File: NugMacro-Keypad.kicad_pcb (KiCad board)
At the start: 2 copper layers, 76.2 x 97.2 mm, 51 parts, among them J2 Conn_01x04, J3 Conn_01x04_Female_For_LCD, SW1 SW_Push, SW2 RotaryEncoder_Switch, U1 ATmega32U4-A, Y1 16MHz

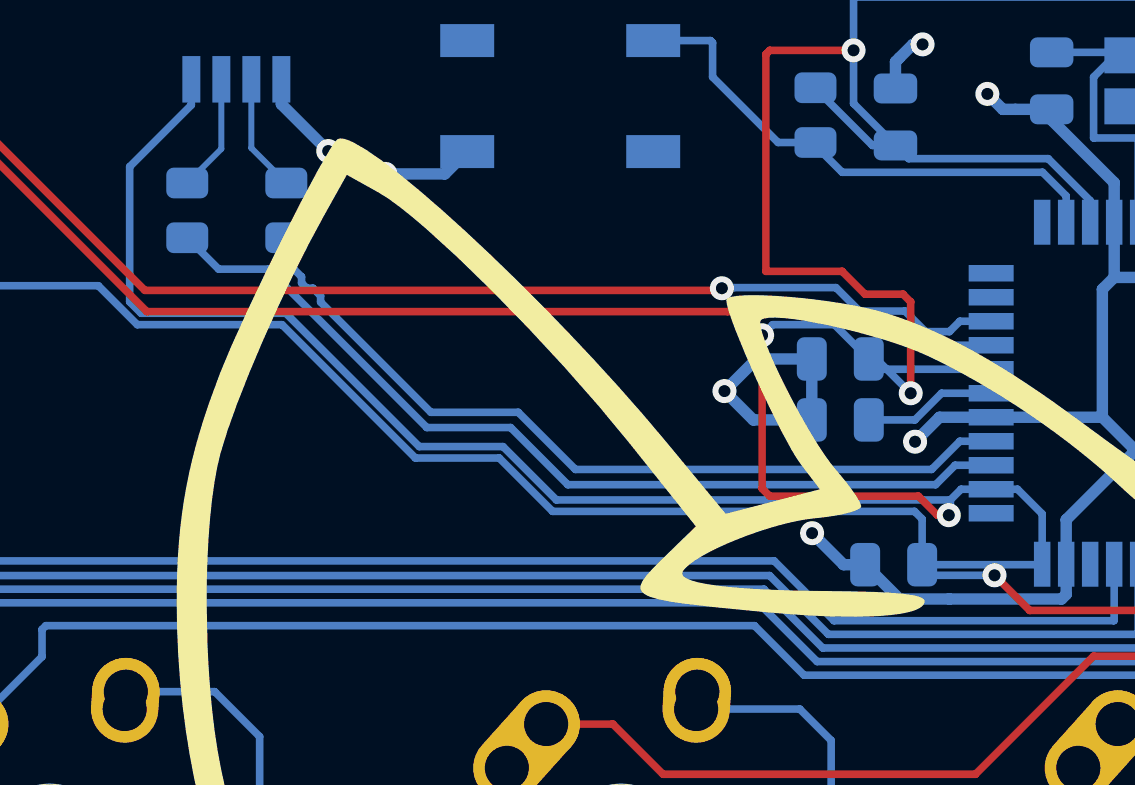
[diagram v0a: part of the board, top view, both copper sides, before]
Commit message: its done
yay
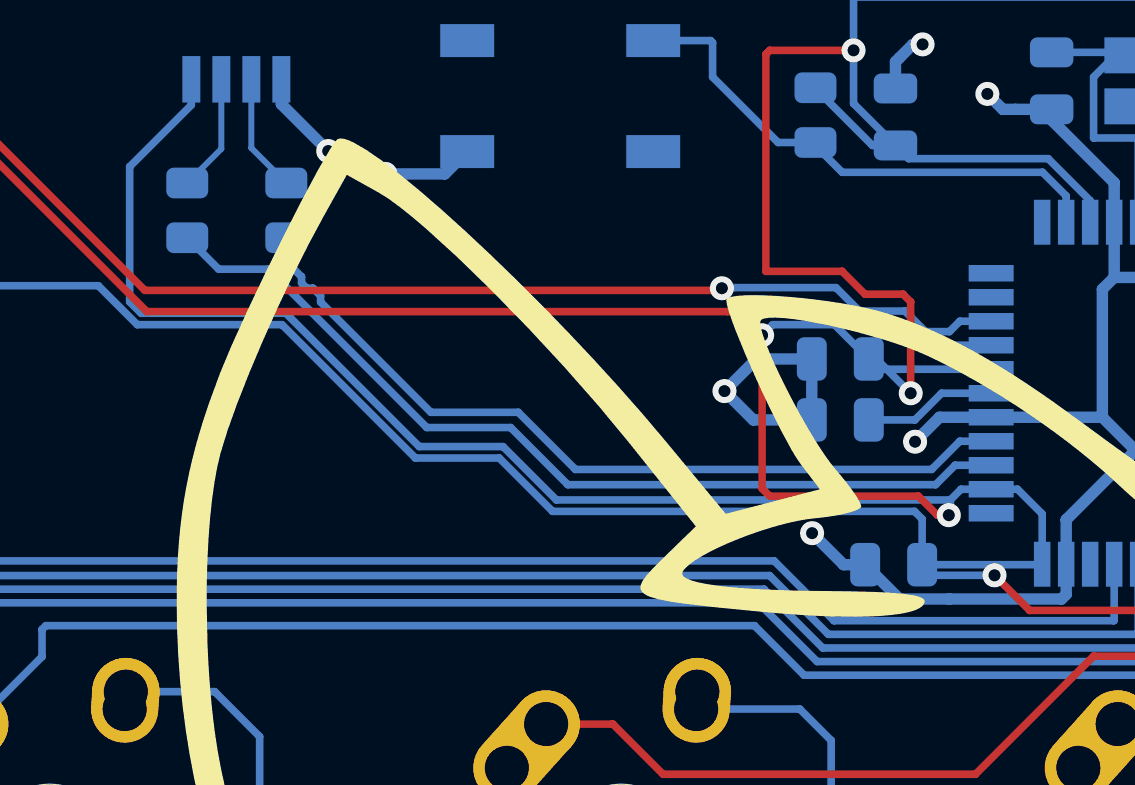
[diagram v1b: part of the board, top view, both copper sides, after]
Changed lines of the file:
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@@
     (title "Nug Macro V3")
     (rev "V3")
-    (company "MIT Liscence")
+    (company "MIT License")
   )
   (layers
@@
   (segment (start 121.6274 48.9834) (end 123.19 50.546) (width 0.381) (layer "B.Cu") (net 2))
   (segment (start 149.3884 54.75847) (end 149.3884 52.91947) (width 0.381) (layer "B.Cu") (net 2))
-  (segment (start 139.3094 59.50847) (end 139.3044 59.51347) (width 0.381) (layer "B.Cu") (net 2))
   (segment (start 147.7884 64.31947) (end 147.7884 62.83547) (width 0.381) (layer "B.Cu") (net 2))
   (segment (start 162.0609 63.06447) (end 162.0609 64.5249) (width 0.381) (layer "B.Cu") (net 2))
@@
   (segment (start 156.63093 68.072) (end 158.877 68.072) (width 0.381) (layer "B.Cu") (net 2))
   (segment (start 159.6854 67.2636) (end 159.6854 66.36647) (width 0.381) (layer "B.Cu") (net 2))
-  (segment (start 143.8935 65.47747) (end 143.891 65.47497) (width 0.381) (layer "B.Cu") (net 2))
   (segment (start 142.0984 48.45947) (end 142.0984 47.57047) (width 0.381) (layer "B.Cu") (net 2))
   (segment (start 149.3884 52.91947) (end 149.3884 51.5984) (width 0.381) (layer "B.Cu") (net 2))
@@
   (segment (start 119.6274 50.47457) (end 118.491 51.61097) (width 0.2) (layer "B.Cu") (net 27))
   (segment (start 119.6274 48.15447) (end 119.6274 50.47457) (width 0.2) (layer "B.Cu") (net 27))
-  (segment (start 118.56903 51.61097) (end 118.3494 51.61097) (width 0.2) (layer "B.Cu") (net 27))
   (segment (start 136.5104 55.89847) (end 136.9454 55.89847) (width 0.254) (layer "F.Cu") (net 28))
   (segment (start 108.204581 49.955405) (end 111.202283 49.955405) (width 0.254) (layer "F.Cu") (net 28))
